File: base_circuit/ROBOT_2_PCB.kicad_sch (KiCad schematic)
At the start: 29 parts, among them J1 Conn_01x04, J2 Output_Supply, J3 Conn_01x01_Female, J4 M1,2, J5 M3,4, M1 Conn_01x04_Female, M2 Conn_01x04_Female, M3 Conn_01x04_Female, M4 Conn_01x04_Female, SW1 SW_SPDT, SW2 SW_SPDT

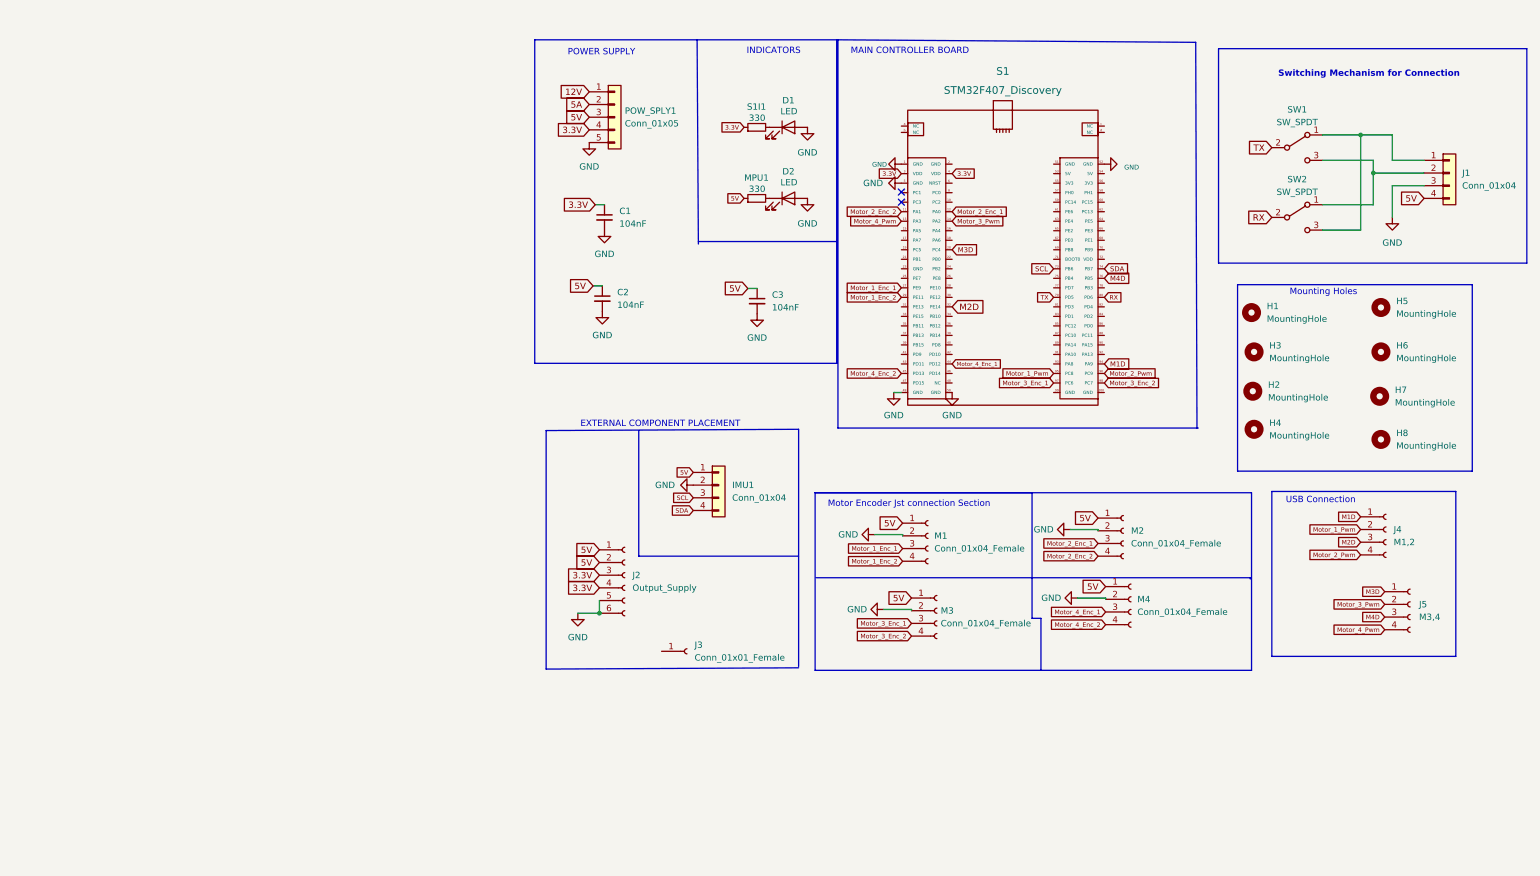
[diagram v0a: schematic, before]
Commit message: Kam vairaxa
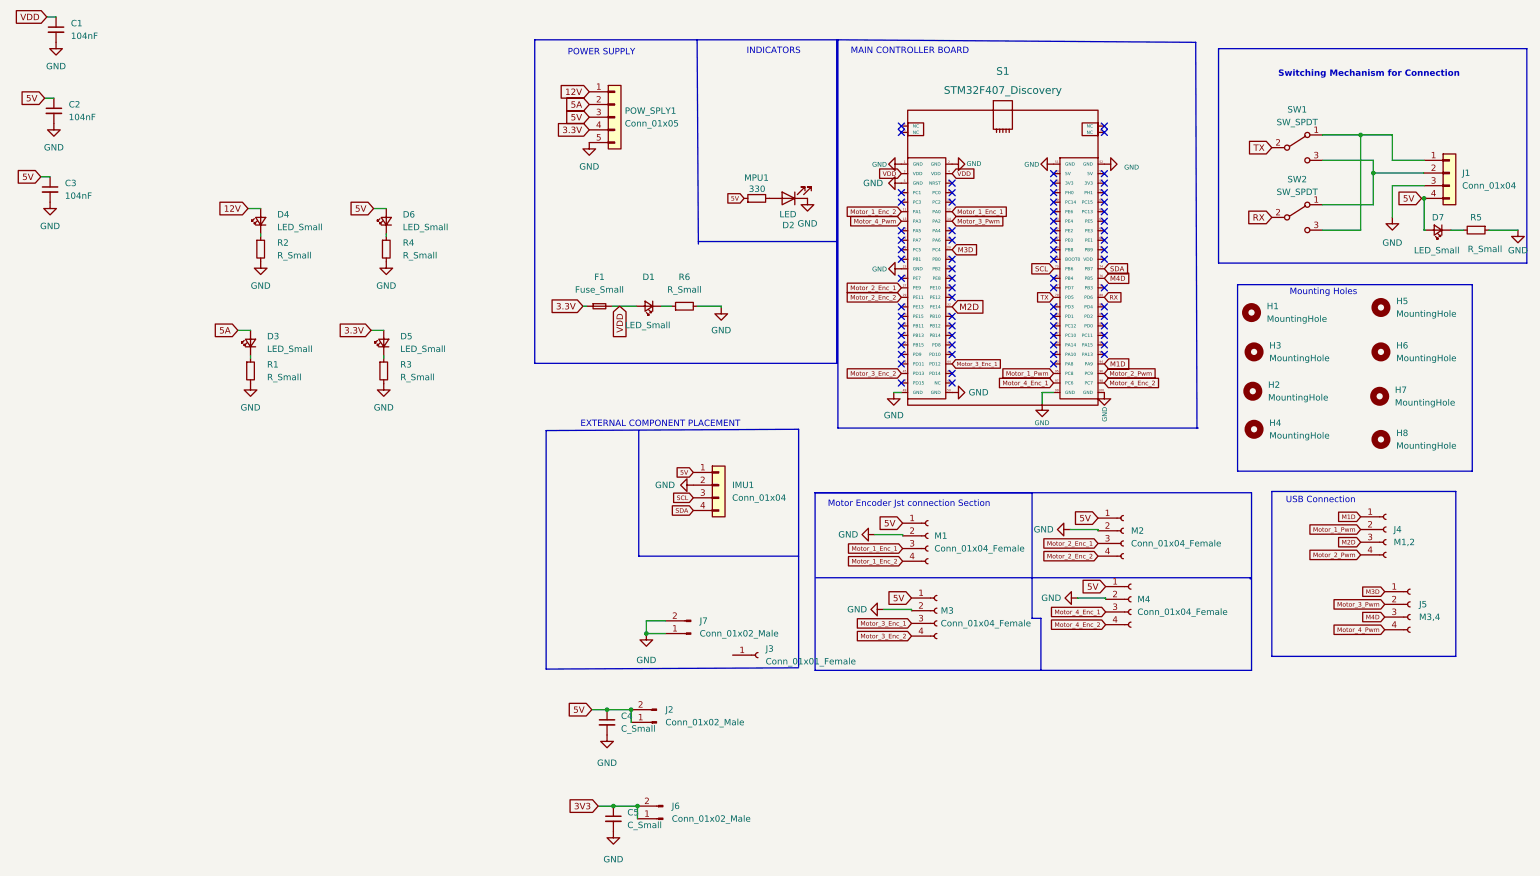
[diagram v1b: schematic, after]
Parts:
- removed D1: LED, modfiles:LED_D3.0mm, symbol Device:LED
- removed J2: Output_Supply, modfiles:JST_5_BIG, symbol Connector:Conn_01x06_Female
- removed S1I1: 330, modfiles:Resistor_small, symbol Device:R_Small
- added C4, C5: C_Small, modfiles:Capacitor_Disc_Small, symbol Device:C_Small
- added D1, D3, D4, D5, D6, D7: LED_Small, modfiles:LED_D3.0mm, symbol Device:LED_Small
- added F1: Fuse_Small, modfiles:Fuse_Holder, symbol Device:Fuse_Small
- added J2, J6, J7: Conn_01x02_Male, modfiles:Connector_Bornier_2, symbol Connector:Conn_01x02_Male
- added R1, R2, R3, R4, R5, R6: R_Small, modfiles:Resistor_small, symbol Device:R_Small
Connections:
- net 12V: now also D4.2 (A)
- net 3.3V: now also D5.2 (A), F1.1; no longer C1.1, S1.3 (VDD), S1.4 (VDD)
- net 5A: now also D3.2 (A)
- net 5V: now also C4.1, D6.2 (A), D7.2 (A), J2.1 (Pin_1), J2.2 (Pin_2)
- net GND: now also D2.1 (K), S1.100 (GND), S1.2 (GND), S1.23 (GND), S1.51 (GND), S1.99 (GND), C4.2, C5.2, J7.1 (Pin_1), J7.2 (Pin_2), R1.2, R2.2, R3.2, R4.2, R5.1, R6.2; no longer D2.2 (A)
- net Motor_1_Enc_1: now also S1.12 (PA0); no longer S1.27 (PE9)
- net Motor_1_Enc_2: now also S1.11 (PA1); no longer S1.29 (PE11)
- net Motor_2_Enc_1: now also S1.27 (PE9); no longer S1.12 (PA0)
- net Motor_2_Enc_2: now also S1.29 (PE11); no longer S1.11 (PA1)
- net Motor_3_Enc_1: now also S1.44 (PD12); no longer S1.97 (PC6)
- net Motor_3_Enc_2: now also S1.45 (PD13); no longer S1.98 (PC7)
- net Motor_4_Enc_1: now also S1.97 (PC6); no longer S1.44 (PD12)
- net Motor_4_Enc_2: now also S1.98 (PC7); no longer S1.45 (PD13)
- net at MPU1.2: now also D2.2 (A); no longer D2.1 (K)
- new net: D1.1 (K), R6.1
- new net: D5.1 (K), R3.1
- new net: D4.1 (K), R2.1
- new net: D7.1 (K), R5.2
- new net: D6.1 (K), R4.1
- new net: D3.1 (K), R1.1
- new net 3V3: C5.1, J6.1 (Pin_1), J6.2 (Pin_2)
- new net VDD: C1.1, D1.2 (A), F1.2, S1.3 (VDD), S1.4 (VDD)
- no-connect marks 2 -> 72
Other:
- moved on the sheet: C1, C2, C3, D2, J3
